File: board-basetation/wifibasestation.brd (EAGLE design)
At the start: 50 x 23 mm, 25 parts, among them J1 SWD_SHROUD_SMD, Q1 MOSFET-PCHANNELSMD

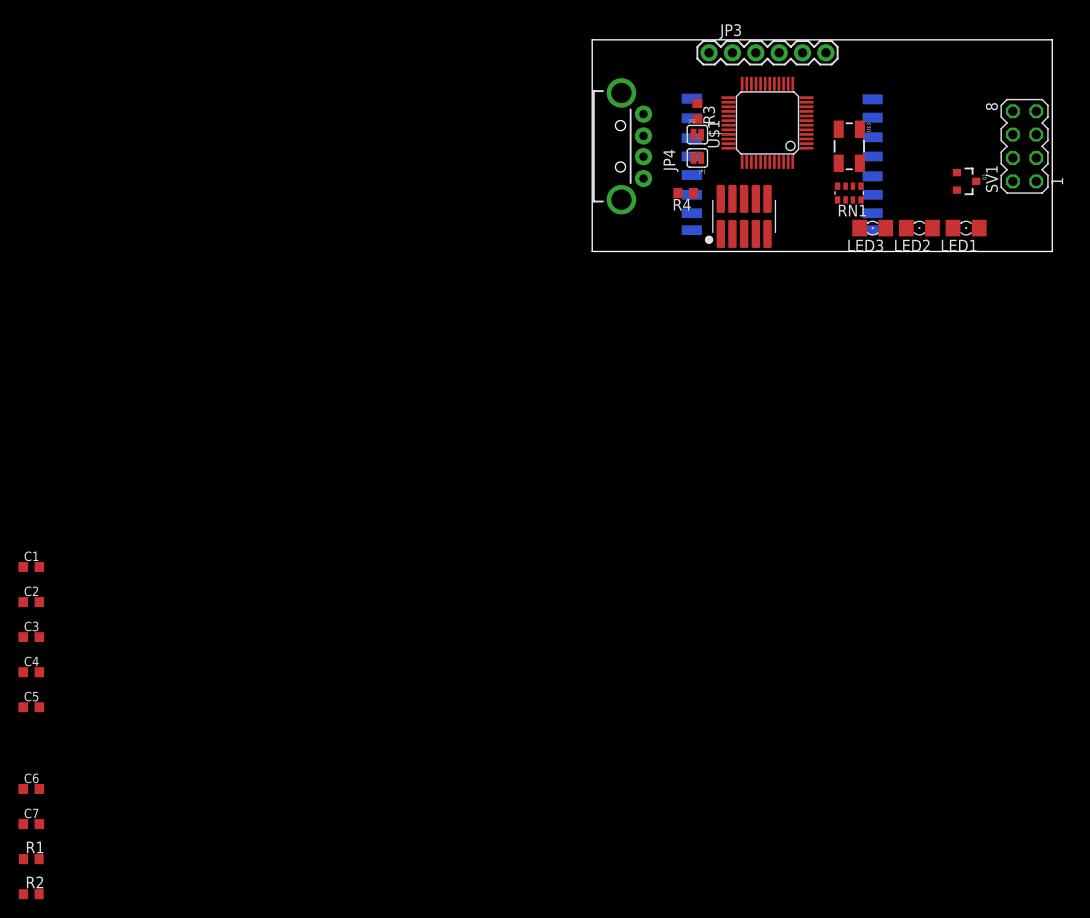
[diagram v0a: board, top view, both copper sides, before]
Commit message: some routing
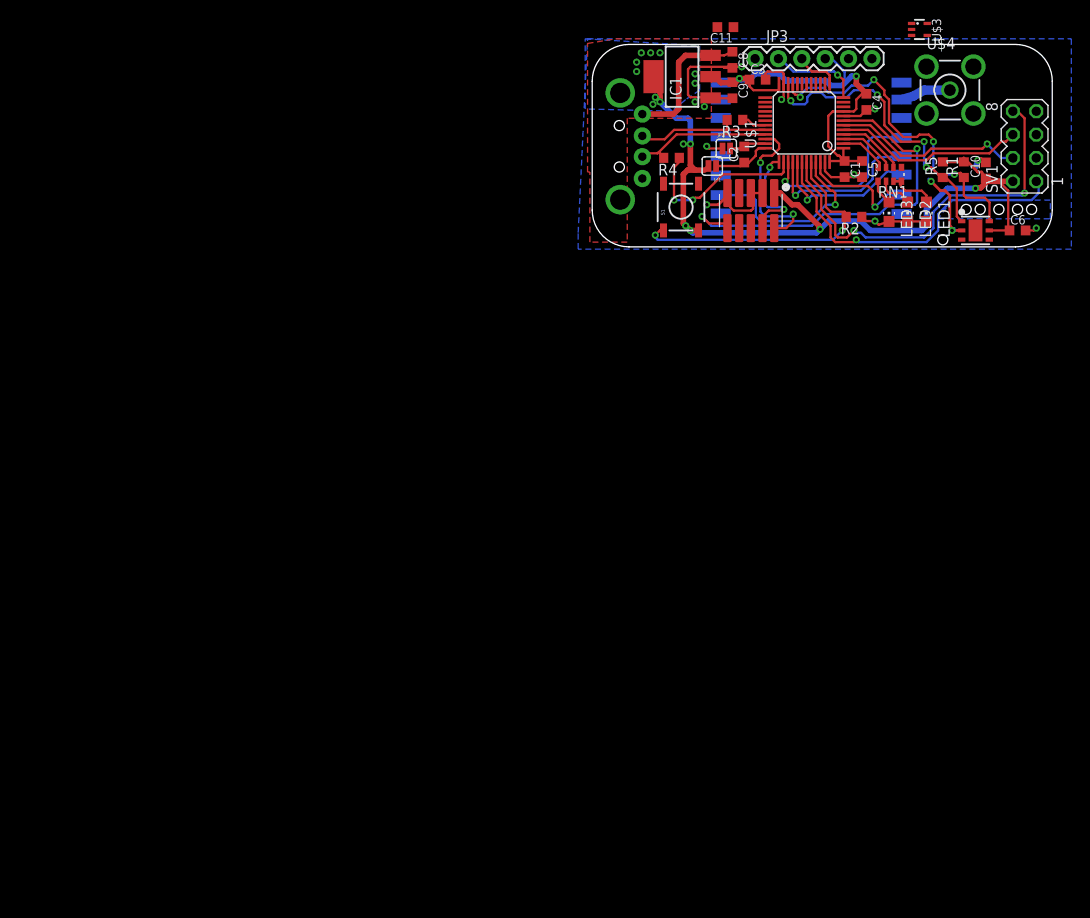
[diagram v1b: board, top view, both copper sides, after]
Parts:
- removed C7: (no value), rcl:C0603K
- removed Q1: MOSFET-PCHANNELSMD, SparkFun-DiscreteSemi:SOT23-3
- added C10, C11, C8, C9: (no value), rcl:C0603K
- added IC1: 1117EMP, dtb:SOT223
- added IC2: HTU21D, Mine:DFN6-L
- added R5: (no value), rcl:R0603
- added S1: SWITCH-MOMENTARY-2SMD, Mine:TACTILE_SWITCH_SMD
- added U$4: BUS-SMA, Ava:BUS-SMA
- LED1, LED2, LED3: device dtb:1206 -> led:CHIP-LED0805
- U$3: value CRYSTAL-GROUNDED -> LMT85; device SparkFun-FreqCtrl:CRYSTAL-SMD-5X3 -> Mine:SC70-5L
- moved R1 126.0 mm to (40.4, 8.89), turned to 90 degrees
- moved C6 123.2 mm to (46.2, 2.29)
- moved R2 115.8 mm to (28.4, 3.76), turned to 180 degrees
- moved C4 109.9 mm to (29.8, 16.3), turned to 270 degrees
- moved C5 107.6 mm to (29.3, 8.95), turned to 270 degrees
- moved C3 99.5 mm to (18.0, 18.7)
- moved C1 98.4 mm to (27.4, 8.95), turned to 270 degrees
- moved C2 91.5 mm to (16.5, 10.5), turned to 90 degrees
- moved U$2 24.5 mm to (14.0, 19.4), turned to 180 degrees
- moved U$3 14.8 mm to (35.6, 24.1)
- moved JP3 5.04 mm to (17.7, 21.0)
- moved RN1 4.84 mm to (32.3, 8.38)
- moved LED1 4.67 mm to (36.3, 4.32)
- moved R3 4.19 mm to (15.5, 14.3), turned to 180 degrees
- moved R4 4.12 mm to (8.62, 10.2)
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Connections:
- removed net N$1: SV1.1
- removed net N$6: SV1.7
- new net CH_PD: SV1.6, U$1.5
- new net DIO0: U$1.45, U$2.DIO0
- new net I2C2_SCL: IC2.6, R1.1, U$1.21
- new net I2C2_SDA: IC2.1, R5.1, U$1.22
- new net MISO: U$1.40, U$2.MISO
- new net MOSI: U$1.41, U$2.MOSI
- new net N$19: U$2.ANT, U$4.1
- new net N$20: LED3.A, RN1.5
- new net N$21: RN1.3, U$1.3
- new net N$22: RN1.2, U$1.4
- new net N$23: U$1.29
- new net N$24: U$1.30
- new net N$26: U$1.26
- new net N$27: U$1.27
- new net NSS: U$1.46, U$2.NSS
- new net RST: U$2.RESET
- new net SCK: U$1.39, U$2.SCK
- new net USART1_RX: SV1.8, U$1.43
- new net USART1_TX: SV1.1, U$1.42
- new net USART2_RX: JP3.TXO, U$1.13
- new net USART2_TX: JP3.RXI, U$1.12
- new net W_RST: SV1.4, U$1.6
- net +3V3: now also C10.1, C11.1, C6.1, C9.1, IC1.2, IC1.4, IC2.5, JP3.VCC, R1.2, R5.2, S1.3, SV1.2, U$2.VCC
- net GND: now also C10.2, C11.2, C8.2, C9.2, IC1.1, IC2.2, JP3.GND, LED1.C, LED2.C, LED3.C, SV1.7, U$2.GNDA, U$2.GNDB, U$4.2, U$4.3, U$4.4, U$4.5; no longer C7.2, U$3.2, U$3.4
- net N$10: now also LED2.A, RN1.6; no longer Q1.2
- net N$12: now also U$1.15; no longer C7.1, R1.2, U$3.3
- net N$14: now also U$1.16; no longer R1.1, U$1.6
- net N$15: now also S1.1
- net N$16: now also U$1.17; no longer C6.1, U$1.5, U$3.1
- net N$2: now also RN1.4, U$1.2; no longer Q1.3, SV1.2
- net N$3: now also U$1.10; no longer SV1.4
- net N$7: now also U$1.11; no longer SV1.6
- net N$8: now also U$1.14; no longer SV1.8
- net N$9: now also LED1.A, RN1.7, RN1.8; no longer Q1.1
- net VBUS: now also C8.1, IC1.3
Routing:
- net +3V3: track 0.00 -> 137.7 mm, vias 0 -> 18
- net GND: track 0.00 -> 65.9 mm, vias 0 -> 13
- net NRST: track 0.00 -> 43.6 mm, vias 0 -> 2
- net USART1_RX: track 0.00 -> 43.3 mm, vias 0 -> 2
- net USART1_TX: track 0.00 -> 37.1 mm, vias 0 -> 1
- net I2C2_SCL: track 0.00 -> 37.1 mm, vias 0 -> 4
- net I2C2_SDA: track 0.00 -> 33.1 mm, vias 0 -> 4
- net N$15: track 0.00 -> 32.4 mm, vias 0 -> 2
- net DIO0: track 0.00 -> 21.1 mm, vias 0 -> 1
- net CH_PD: track 0.00 -> 21.0 mm
- net W_RST: track 0.00 -> 20.9 mm, vias 0 -> 1
- net SCK: track 0.00 -> 19.6 mm, vias 0 -> 1
- net N$18: track 0.00 -> 19.5 mm, vias 0 -> 2
- net MISO: track 0.00 -> 18.0 mm, vias 0 -> 1
- net SWDAT: track 0.00 -> 17.6 mm, vias 0 -> 2
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- added copper zone on layer 1, net +3V3
- added copper zone on layer 16, net +3V3
- added copper zone on layer 16, net GND
- added copper zone on layer 16, net N$1
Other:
- board size 50 x 23 mm -> 50 x 22 mm
